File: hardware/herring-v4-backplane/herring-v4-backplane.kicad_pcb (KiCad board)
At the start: 4 copper layers, 100 x 100 mm, 33 parts, among them J1 Conn_02x20_Odd_Even, J2 Conn_02x10_Odd_Even, J3 Conn_02x20_Odd_Even, J4 Conn_02x10_Odd_Even, J5 Conn_02x20_Odd_Even, J6 Conn_02x10_Odd_Even, J7 Conn_02x20_Odd_Even, J8 Conn_02x10_Odd_Even, J9 Jack-DC, SW1 SW_Push, SW2 SW_SPDT, U1 NE555P

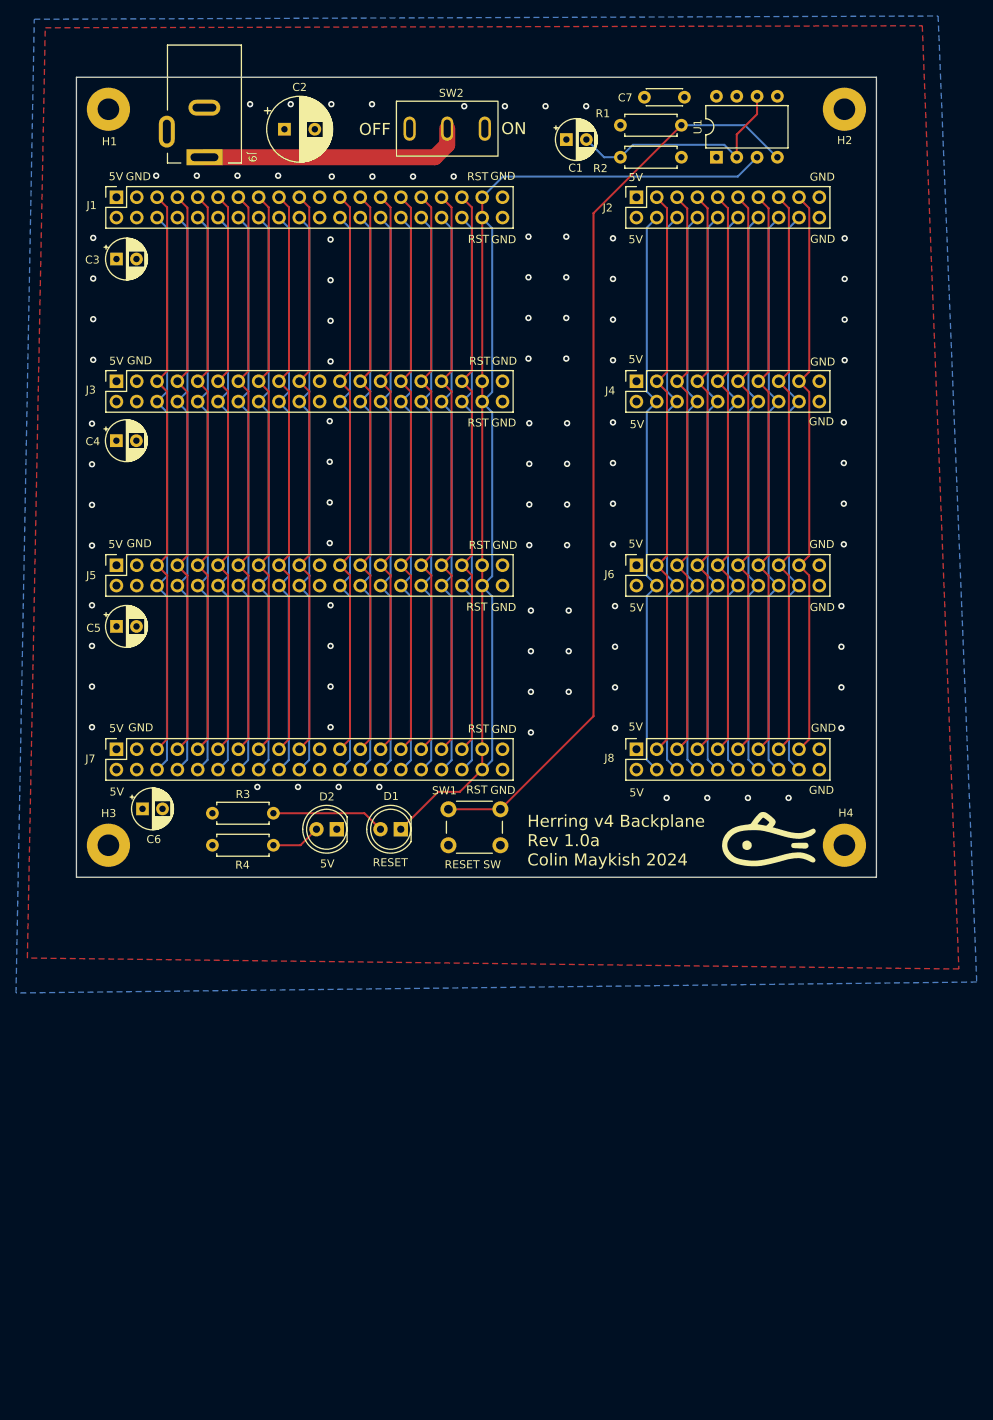
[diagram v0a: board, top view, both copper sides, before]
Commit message: herring v4 backplane routed
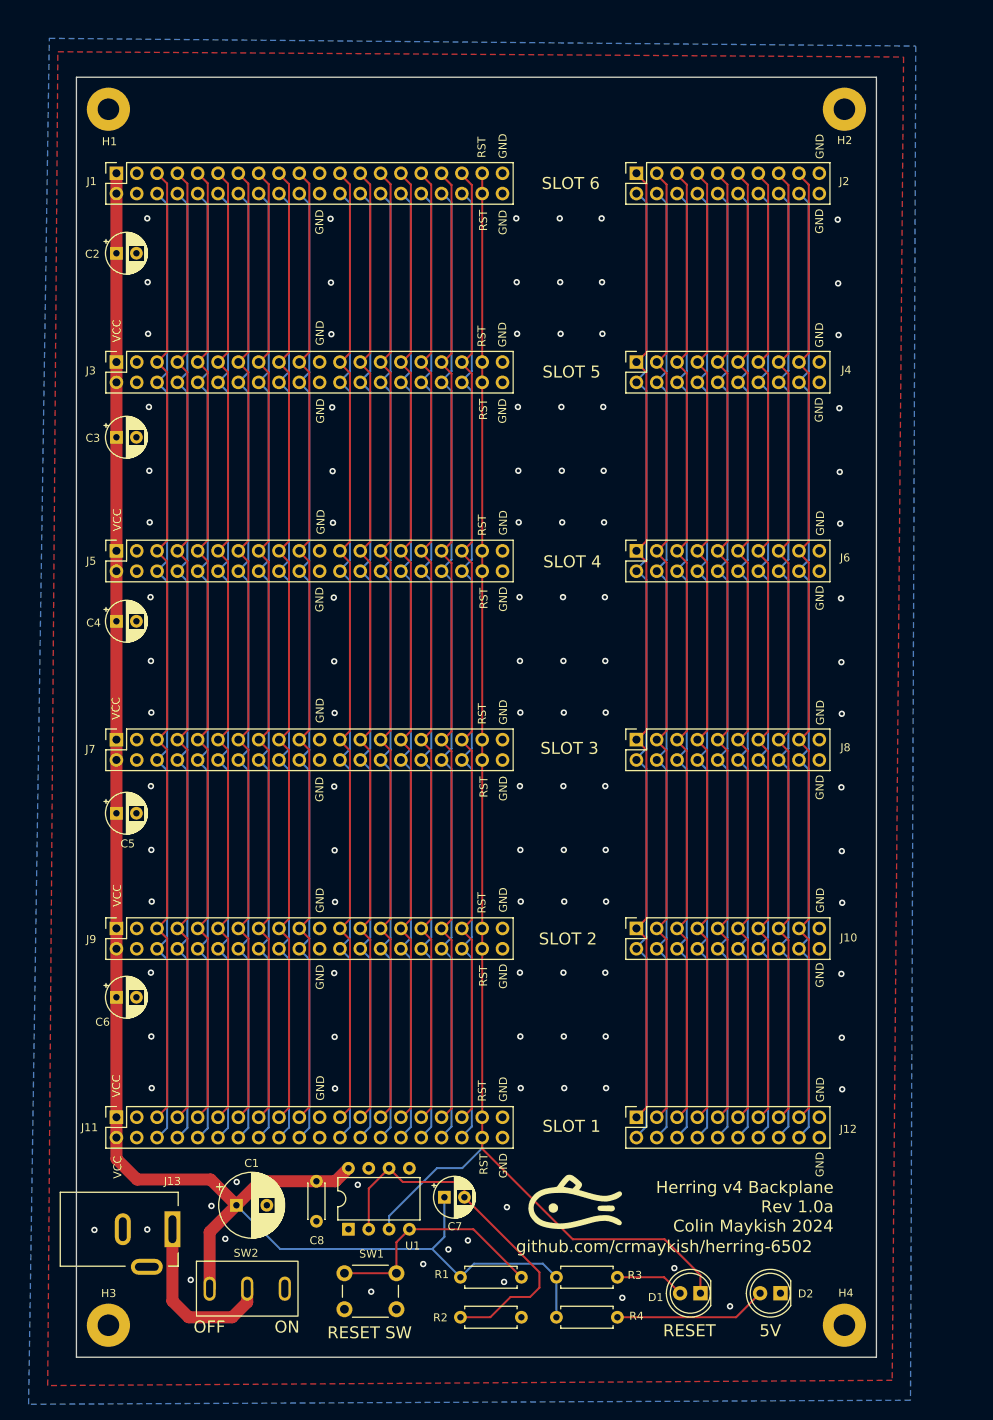
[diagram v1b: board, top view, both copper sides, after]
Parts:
- removed the G*** at (78.0, 95.8)
- removed the G*** at (93.4, 95.8)
- removed the G*** at (108.3, 95.8)
- added C6: C_Polarized_US, Capacitor_THT:CP_Radial_D5.0mm_P2.50mm, F.Cu at (25.0, 135.0)
- added J10: Conn_02x10_Odd_Even, Connector_PinSocket_2.54mm:PinSocket_2x10_P2.54mm_Vertical, F.Cu at (90.0, 126.4)
- added J11: Conn_02x20_Odd_Even, Connector_PinSocket_2.54mm:PinSocket_2x20_P2.54mm_Vertical, F.Cu at (25.0, 150.0)
- added J12: Conn_02x10_Odd_Even, Connector_PinSocket_2.54mm:PinSocket_2x10_P2.54mm_Vertical, F.Cu at (90.0, 150.0)
- added J9: Conn_02x20_Odd_Even, Connector_PinSocket_2.54mm:PinSocket_2x20_P2.54mm_Vertical, F.Cu at (25.0, 126.4)
- moved SW2 147.1 mm to (35.0, 168.0)
- moved R2 146.4 mm to (68.0, 175.0)
- moved R1 145.4 mm to (68.0, 170.0)
- moved C8 143.1 mm to (50.0, 158.0), turned to -90 degrees
- moved U1 141.7 mm to (54.0, 164.0)
- moved C1 134.6 mm to (40.0, 161.0)
- moved J13 134.1 mm to (32.0, 164.0), turned to 0 degrees
- moved C7 133.1 mm to (66.0, 160.0)
- moved D2 80.2 mm to (108.0, 172.0)
- moved R4 73.0 mm to (80.0, 175.0)
- moved R3 72.2 mm to (80.0, 170.0)
- moved D1 69.0 mm to (98.0, 172.0)
- moved H3 60.0 mm to (24.0, 176.0)
- moved H4 60.0 mm to (116.0, 176.0)
- moved SW1 59.4 mm to (60.0, 174.0)
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- renumbered C2 to C1, C3 to C2, C4 to C3, C5 to C4, C6 to C5, C1 to C7, C7 to C8, J9 to J13
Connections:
- J2 pad 1: +5V -> /B48
- J2 pad 2: +5V -> /B49
- J4 pad 1: +5V -> /B48
- J4 pad 2: +5V -> /B49
- J6 pad 1: +5V -> /B48
- J6 pad 2: +5V -> /B49
- J8 pad 1: +5V -> /B48
- J8 pad 2: +5V -> /B49
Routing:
- net +5V: track 0.00 -> 225.2 mm
- net /B48: track 0.00 -> 123.2 mm
- net /B49: track 0.00 -> 123.2 mm
- net Net-(R1-Pad2): track 115.0 -> 29.2 mm
- net /B46: track 72.1 -> 123.2 mm
- net /B38: track 72.1 -> 123.2 mm
- net /B30: track 72.1 -> 123.2 mm
- net /B14: track 72.1 -> 123.2 mm
- net /B10: track 72.1 -> 123.2 mm
- net /B27: track 72.1 -> 123.2 mm
- net /B24: track 72.1 -> 123.2 mm
- net /B19: track 72.1 -> 123.2 mm
- net /B18: track 72.1 -> 123.2 mm
- net /B11: track 72.1 -> 123.2 mm
- net /B1: track 72.1 -> 123.2 mm
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- removed copper zone on In2.Cu, net +5V
- removed copper zone on In1.Cu, net GND
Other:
- board size 100 x 100 mm -> 100 x 160 mm
- copper layers 4 -> 2
- board text added: "SLOT 1"
- board text added: "SLOT 2"
- board text added: "SLOT 3"
- board text added: "SLOT 4"
- board text added: "SLOT 5"
- board text added: "SLOT 6"
- board text added: "VCC"
